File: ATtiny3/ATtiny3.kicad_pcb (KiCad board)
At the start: 2 copper layers, 87.6 x 31.8 mm, 48 parts, among them J1 LEDOUT1, J2 LEDOUT1, J3 POWER, Q1 SMD-MOSFET-N-CH-20V-2.1A-CJ23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, Q2 SMD-MOSFET-N-CH-20V-2.1A-CJ23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, Q3 SMD-MOSFET-N-CH-20V-2.1A-CJ23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, Q4 SMD-MOSFET-N-CH-20V-2.1A-CJ23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, Q5 SMD-MOSFET-N-CH-20V-2.1A-CJ23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, Q6 SMD-MOSFET-N-CH-20V-2.1A-CJ23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, Q7 SMD-MOSFET-N-CH-20V-2.1A-CJ23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, Q8 SMD-MOSFET-N-CH-20V-2.1A-CJ23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, U1 ATtiny824-X, U2 AP2127K-3.3

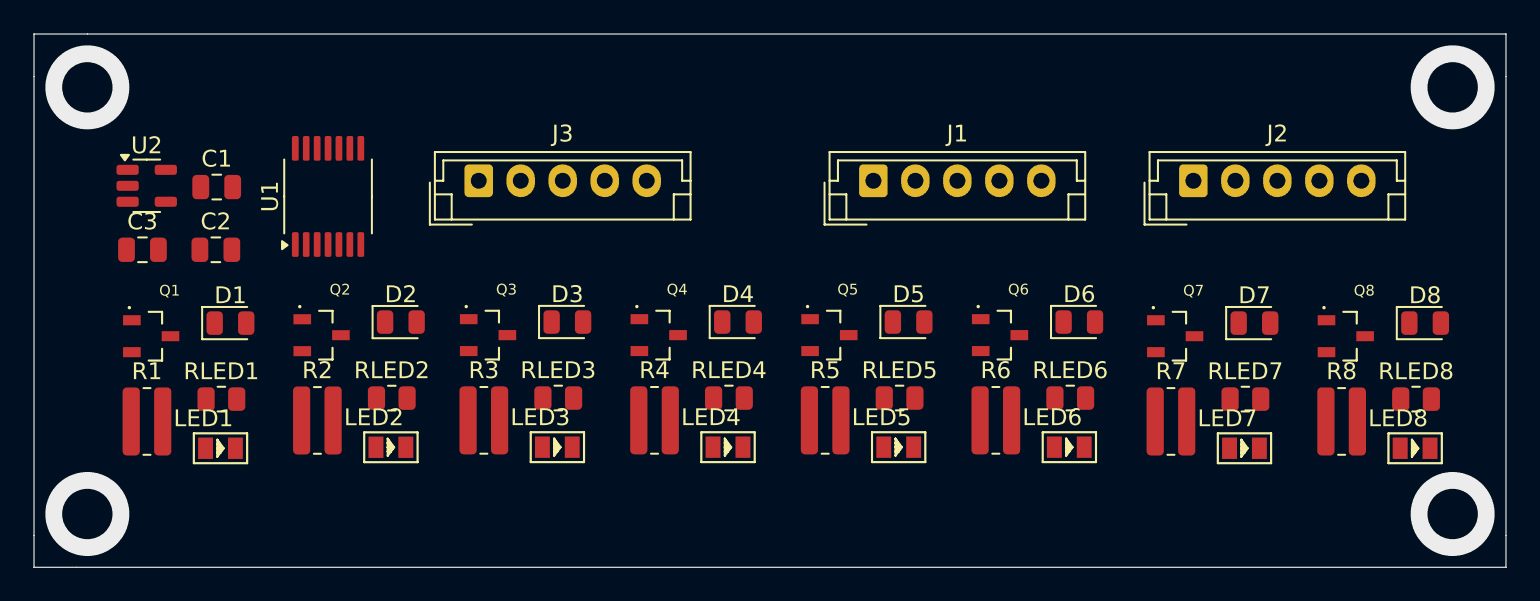
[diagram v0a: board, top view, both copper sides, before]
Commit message: Primo ordine JLCPCB
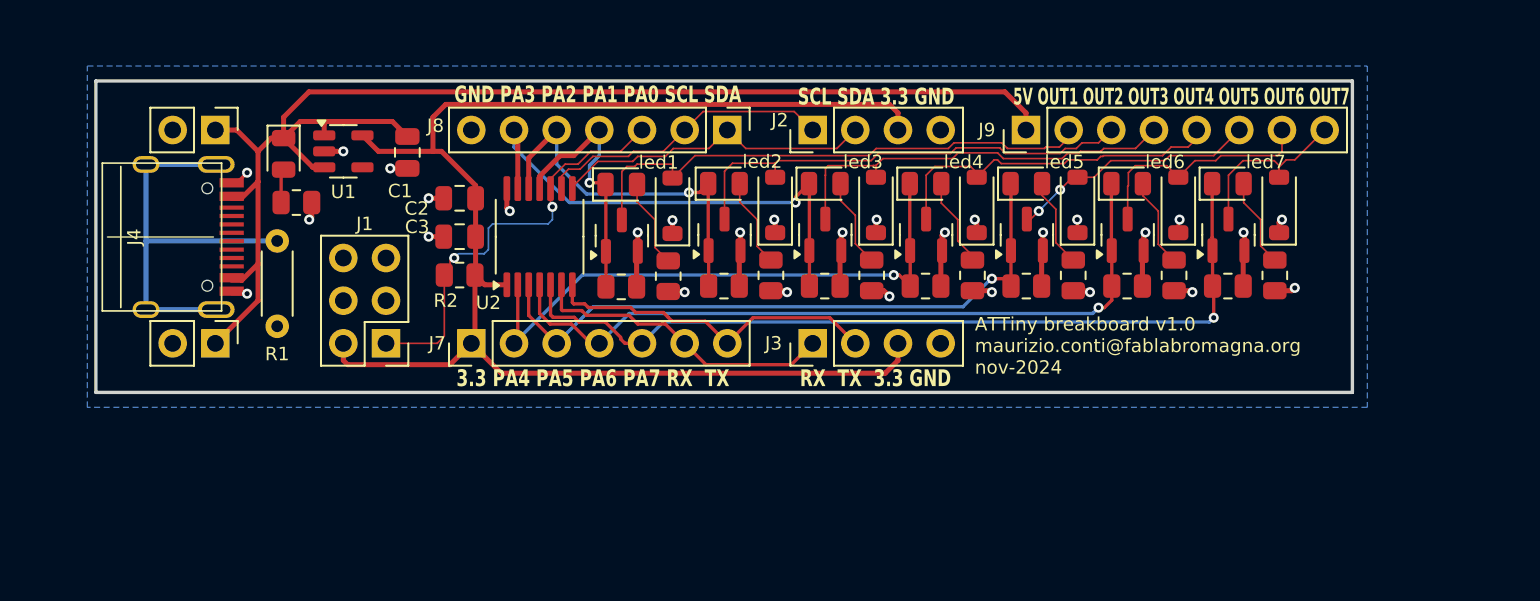
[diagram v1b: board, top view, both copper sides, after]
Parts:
- removed D1, D2, D3, D4, D5, D6, D7, D8: SMD-DIODE-SCHOTTKY-20V-1A_SOD-123_, Diode_SMD:D_0805_2012Metric
- removed LED1, LED2, LED3, LED4, LED5, LED6, LED7, LED8: SMD-LED-CLEAR-RED_0805_, Library:LED-0805
- removed Q1, Q2, Q3, Q4, Q5, Q6, Q7, Q8: SMD-MOSFET-N-CH-20V-2.1A-CJ2302_SOT-23_, Library:SOT95P240X115-3N
- removed R3, R4, R5, R6, R7, R8: SMD-RES-4.7K-5%-1_8W_0805_, Resistor_SMD:R_0815_2038Metric
- removed RLED1, RLED2, RLED3, RLED4, RLED5, RLED6, RLED7, RLED8: SMD-RES-220R-5%-1_8W_0805_, Resistor_SMD:R_0805_2012Metric
- added J4: USB_C_Receptacle_USB2.0_16P, Library-USB:TYPE-C-31-M-12, F.Cu at (21.3, 29.2)
- added J5: MNT01, Connector_PinHeader_2.54mm:PinHeader_1x02_P2.54mm_Vertical, F.Cu at (25.4, 35.6)
- added J6: MNT02, Connector_PinHeader_2.54mm:PinHeader_1x02_P2.54mm_Vertical, F.Cu at (25.4, 22.9)
- added J7: ATTiny1, Connector_PinHeader_2.54mm:PinHeader_1x07_P2.54mm_Vertical, F.Cu at (40.6, 35.6)
- added J8: ATTiny1, Connector_PinHeader_2.54mm:PinHeader_1x07_P2.54mm_Vertical, F.Cu at (55.9, 22.9)
- added J9: LEDOUT1, Connector_PinHeader_2.54mm:PinHeader_1x08_P2.54mm_Vertical, F.Cu at (73.7, 22.9)
- added L1: Logo_Open_Hardware_Small, Symbol:OSHW-Logo_5.7x6mm_SilkScreen, B.Cu at (42.3, 28.7)
- added LedON1: SMD-LED-CLEAR-RED_0805_, LED_SMD:LED_0805_2012Metric, F.Cu at (29.5, 24.3)
- added RLedON1: SMD-RES-220R-5%-1_8W_0805_, Resistor_SMD:R_0805_2012Metric, F.Cu at (30.2, 27.2)
- added dq1: SMD-DIODE-SCHOTTKY-20V-1A_SOD-123_, Diode_SMD:D_SOD-123, F.Cu at (52.6, 27.4)
- added dq2: SMD-DIODE-SCHOTTKY-20V-1A_SOD-123_, Diode_SMD:D_SOD-123, F.Cu at (58.7, 27.3)
- added dq3: SMD-DIODE-SCHOTTKY-20V-1A_SOD-123_, Diode_SMD:D_SOD-123, F.Cu at (64.7, 27.3)
- added dq4: SMD-DIODE-SCHOTTKY-20V-1A_SOD-123_, Diode_SMD:D_SOD-123, F.Cu at (70.7, 27.3)
- added dq5: SMD-DIODE-SCHOTTKY-20V-1A_SOD-123_, Diode_SMD:D_SOD-123, F.Cu at (76.7, 27.3)
- added dq6: SMD-DIODE-SCHOTTKY-20V-1A_SOD-123_, Diode_SMD:D_SOD-123, F.Cu at (82.7, 27.3)
- added dq7: SMD-DIODE-SCHOTTKY-20V-1A_SOD-123_, Diode_SMD:D_SOD-123, F.Cu at (88.7, 27.3)
- added led1: SMD-LED-CLEAR-0805, LED_SMD:LED_0805_2012Metric, F.Cu at (49.6, 26.1)
- added led2: SMD-LED-CLEAR-0805, LED_SMD:LED_0805_2012Metric, F.Cu at (55.7, 26.1)
- added led3: SMD-LED-CLEAR-0805, LED_SMD:LED_0805_2012Metric, F.Cu at (61.7, 26.1)
- added led4: SMD-LED-CLEAR-0805, LED_SMD:LED_0805_2012Metric, F.Cu at (67.7, 26.1)
- added led5: SMD-LED-CLEAR-0805, LED_SMD:LED_0805_2012Metric, F.Cu at (73.7, 26.1)
- added led6: SMD-LED-CLEAR-0805, LED_SMD:LED_0805_2012Metric, F.Cu at (79.7, 26.1)
- added led7: SMD-LED-CLEAR-0805, LED_SMD:LED_0805_2012Metric, F.Cu at (85.7, 26.1)
- added q1: SMD-MOSFET-N-CH, Package_TO_SOT_SMD:SOT-23, F.Cu at (49.6, 29.1)
- added q2: SMD-MOSFET-N-CH, Package_TO_SOT_SMD:SOT-23, F.Cu at (55.7, 29.1)
- added q3: SMD-MOSFET-N-CH, Package_TO_SOT_SMD:SOT-23, F.Cu at (61.7, 29.1)
- added q4: SMD-MOSFET-N-CH, Package_TO_SOT_SMD:SOT-23, F.Cu at (67.7, 29.1)
- added q5: SMD-MOSFET-N-CH, Package_TO_SOT_SMD:SOT-23, F.Cu at (73.7, 29.1)
- added q6: SMD-MOSFET-N-CH, Package_TO_SOT_SMD:SOT-23, F.Cu at (79.7, 29.1)
- added q7: SMD-MOSFET-N-CH, Package_TO_SOT_SMD:SOT-23, F.Cu at (85.7, 29.1)
- added rgate1: 10K, Resistor_SMD:R_0805_2012Metric, F.Cu at (49.6, 32.2)
- added rgate2: 10K, Resistor_SMD:R_0805_2012Metric, F.Cu at (55.7, 32.1)
- added rgate3: 10K, Resistor_SMD:R_0805_2012Metric, F.Cu at (61.7, 32.1)
- added rgate4: 10K, Resistor_SMD:R_0805_2012Metric, F.Cu at (67.7, 32.1)
- added rgate5: 10K, Resistor_SMD:R_0805_2012Metric, F.Cu at (73.7, 32.1)
- added rgate6: 10K, Resistor_SMD:R_0805_2012Metric, F.Cu at (79.7, 32.1)
- added rgate7: 10K, Resistor_SMD:R_0805_2012Metric, F.Cu at (85.7, 32.1)
- added rled1: SMD-RES-220R-5%-1_8W_0805_, Resistor_SMD:R_0805_2012Metric, F.Cu at (52.4, 31.6)
- added rled2: SMD-RES-220R-5%-1_8W_0805_, Resistor_SMD:R_0805_2012Metric, F.Cu at (58.5, 31.5)
- added rled3: SMD-RES-220R-5%-1_8W_0805_, Resistor_SMD:R_0805_2012Metric, F.Cu at (64.5, 31.5)
- added rled4: SMD-RES-220R-5%-1_8W_0805_, Resistor_SMD:R_0805_2012Metric, F.Cu at (70.5, 31.5)
- added rled5: SMD-RES-220R-5%-1_8W_0805_, Resistor_SMD:R_0805_2012Metric, F.Cu at (76.5, 31.5)
- added rled6: SMD-RES-220R-5%-1_8W_0805_, Resistor_SMD:R_0805_2012Metric, F.Cu at (82.5, 31.5)
- added rled7: SMD-RES-220R-5%-1_8W_0805_, Resistor_SMD:R_0805_2012Metric, F.Cu at (88.5, 31.5)
- J1: value LEDOUT1 -> UPDI; footprint Connector_JST:JST_EH_B5B-EH-A_1x05_P2.50mm_Vertical -> Connector_PinHeader_2.54mm:PinHeader_2x03_P2.54mm_Vertical
- J2: value LEDOUT1 -> I2C; footprint Connector_JST:JST_EH_B5B-EH-A_1x05_P2.50mm_Vertical -> Connector_PinHeader_2.54mm:PinHeader_1x04_P2.54mm_Vertical
- J3: value POWER -> Serial; footprint Connector_JST:JST_EH_B5B-EH-A_1x05_P2.50mm_Vertical -> Connector_PinHeader_2.54mm:PinHeader_1x04_P2.54mm_Vertical
- R1: value SMD-RES-4.7K-5%-1_8W_0805_ -> 1M; footprint Resistor_SMD:R_0815_2038Metric -> Resistor_THT:R_Axial_DIN0204_L3.6mm_D1.6mm_P5.08mm_Horizontal
- R2: value SMD-RES-4.7K-5%-1_8W_0805_ -> 10K; footprint Resistor_SMD:R_0815_2038Metric -> Resistor_SMD:R_0805_2012Metric
- U1: value ATtiny824-X -> AP2127K-3.3; footprint Package_SO:TSSOP-14_4.4x5mm_P0.65mm -> Package_TO_SOT_SMD:SOT-23-5
- U2: value AP2127K-3.3 -> ATtiny824-X; footprint Package_TO_SOT_SMD:SOT-23-5 -> Package_SO:TSSOP-14_4.4x5mm_P0.65mm
- moved J1 30.6 mm to (35.6, 35.6), turned to 180 degrees
- moved U2 23.6 mm to (44.7, 29.2), turned to 90 degrees
- moved J2 22.9 mm to (61.0, 22.9), turned to 90 degrees
- moved J3 22.1 mm to (61.0, 35.6), turned to 90 degrees
- moved C1 16.8 mm to (36.8, 24.2), turned to -90 degrees
- moved C3 14.5 mm to (39.9, 29.2), turned to 180 degrees
- moved C2 14.5 mm to (39.9, 26.9), turned to 180 degrees
- moved R1 13.3 mm to (29.1, 29.5), turned to -90 degrees
- moved R2 12.1 mm to (39.9, 31.5), turned to 180 degrees
- moved U1 2.83 mm to (33.0, 24.1), turned to 0 degrees
- renumbered C3 to C1, C1 to C2, C2 to C3
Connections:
- J1 pad 1: +5V -> PA0-UPDI
- J1 pad 2: /Mosfet Driver 4/_OUT -> +3.3V
- J1 pad 3: /Mosfet Driver 3/_OUT -> unconnected-(J1-Pin_3-Pad3)
- J1 pad 4: /Mosfet Driver 2/_OUT -> unconnected-(J1-Pin_4-Pad4)
- J1 pad 5: /Mosfet Driver 1/_OUT -> unconnected-(J1-Pin_5-Pad5)
- J2 pad 1: +5V -> PB0-SCL
- J2 pad 2: /Mosfet Driver 8/_OUT -> PB1-SDA
- J2 pad 3: /Mosfet Driver 7/_OUT -> +3.3V
- J2 pad 4: /Mosfet Driver 6/_OUT -> GND
- J3 pad 1: +5V -> PB3-RX
- J3 pad 2: GND -> PB2-TX
- J3 pad 3: GND -> +3.3V
- J3 pad 4: UPDI -> GND
- R1 pad 1: /Mosfet Driver 2/_IN -> Net-(J4-SHIELD)
- R2 pad 1: /Mosfet Driver 1/_IN -> +3.3V
- R2 pad 2: GND -> PA0-UPDI
- U1 pad 1: +3.3V -> +5V
- U1 pad 2: /Mosfet Driver 4/_IN -> GND
- U1 pad 3: /Mosfet Driver 5/_IN -> +5V
- U1 pad 4: /Mosfet Driver 6/_IN -> unconnected-(U1-NC-Pad4)
- U1 pad 5: /Mosfet Driver 7/_IN -> +3.3V
- U2 pad 1: +5V -> +3.3V
- U2 pad 2: GND -> PA4
- U2 pad 3: +5V -> PA5
- U2 pad 4: unconnected-(U2-NC-Pad4) -> PA6
- U2 pad 5: +3.3V -> PA7
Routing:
- net +3.3V: track 0.00 -> 87.6 mm
- net +5V: track 0.00 -> 81.1 mm
- net PA7: track 0.00 -> 51.2 mm, vias 0 -> 1
- net GND: track 0.00 -> 44.8 mm, vias 0 -> 29
- net PA6: track 0.00 -> 44.5 mm, vias 0 -> 1
- net PA5: track 0.00 -> 39.1 mm, vias 0 -> 1
- net PA4: track 0.00 -> 35.2 mm, vias 0 -> 1
- net OUT1: track 0.00 -> 32.2 mm
- net PA3: track 0.00 -> 30.3 mm, vias 0 -> 1
- net OUT2: track 0.00 -> 28.1 mm
- net PA0-UPDI: track 0.00 -> 25.4 mm, vias 0 -> 2
- net Net-(J4-SHIELD): track 0.00 -> 24.8 mm
- net OUT3: track 0.00 -> 24.5 mm
- net PA2: track 0.00 -> 22.4 mm, vias 0 -> 1
- net OUT4: track 0.00 -> 21.0 mm
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- added copper zone on B.Cu, net GND
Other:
- board size 87.6 x 31.8 mm -> 74.8 x 18.5 mm
- board text added: "3.3 PA4 PA5 PA6 PA7 RX TX"
- board text added: "5V OUT1 OUT2 OUT3 OUT4 OUT5 OUT6 OUT7"
- board text added: "ATTiny breakboard v1.0 maurizio.conti@fablabromagna.org nov-2024"
- board text added: "GND PA3 PA2 PA1 PA0 SCL SDA"
- board text added: "RX TX 3.3 GND"
- board text added: "SCL SDA 3.3 GND"
